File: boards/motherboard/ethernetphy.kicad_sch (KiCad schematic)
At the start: 25 parts, among them U5 DP83848I, X1 50M

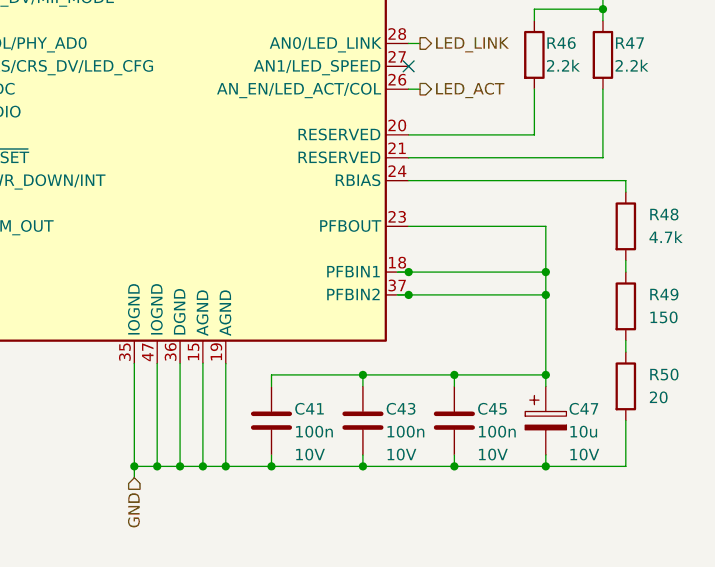
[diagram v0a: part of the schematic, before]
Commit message: feat: finalizing up schematic
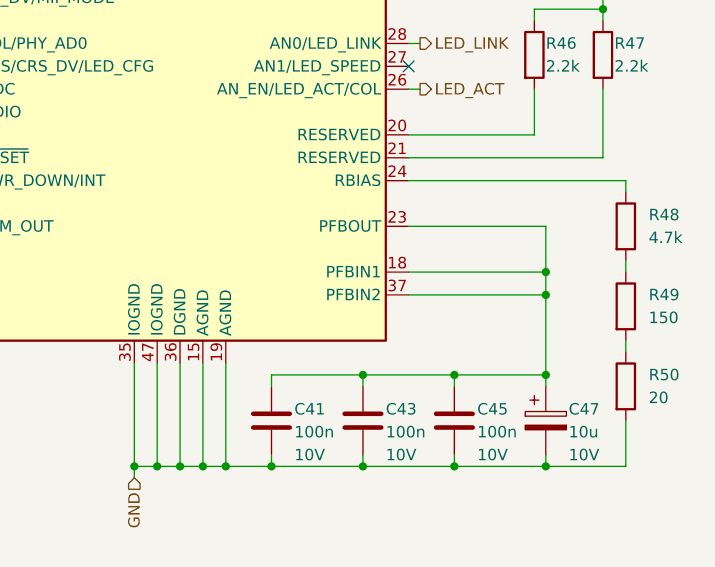
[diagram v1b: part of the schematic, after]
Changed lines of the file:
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@@
   (junction (at 124.46 149.86) (diameter 0) (color 0 0 0 0)
   )
-  (junction (at 129.54 130.81) (diameter 0) (color 0 0 0 0)
-  )
   (junction (at 121.92 40.64) (diameter 0) (color 0 0 0 0)
   )
@@
   )
   (junction (at 48.26 105.41) (diameter 0) (color 0 0 0 0)
-  )
-  (junction (at 129.54 128.27) (diameter 0) (color 0 0 0 0)
   )
   (junction (at 104.14 40.64) (diameter 0) (color 0 0 0 0)
@@
     (stroke (width 0) (type default) (color 0 0 0 0))
   )
-  (wire (pts (xy 128.27 130.81) (xy 129.54 130.81))
-    (stroke (width 0) (type default) (color 0 0 0 0))
-  )
   (wire (pts (xy 109.22 138.43) (xy 109.22 149.86))
     (stroke (width 0) (type default) (color 0 0 0 0))
@@
     (stroke (width 0) (type default) (color 0 0 0 0))
   )
-  (wire (pts (xy 128.27 128.27) (xy 129.54 128.27))
-    (stroke (width 0) (type default) (color 0 0 0 0))
-  )
